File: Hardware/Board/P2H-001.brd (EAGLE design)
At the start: 47 x 72 mm, 14 parts, among them IC1 74LS07N, IC2 LTC485N

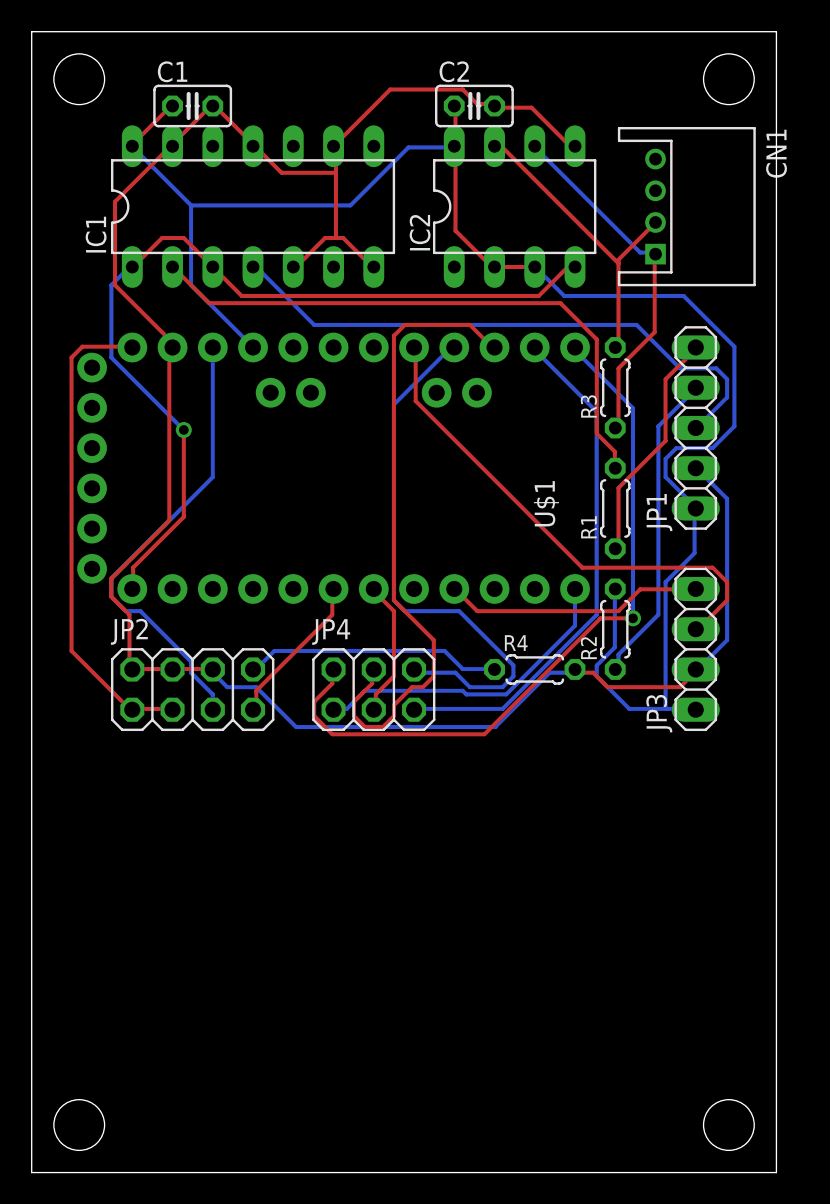
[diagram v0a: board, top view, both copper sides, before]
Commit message: New board design.
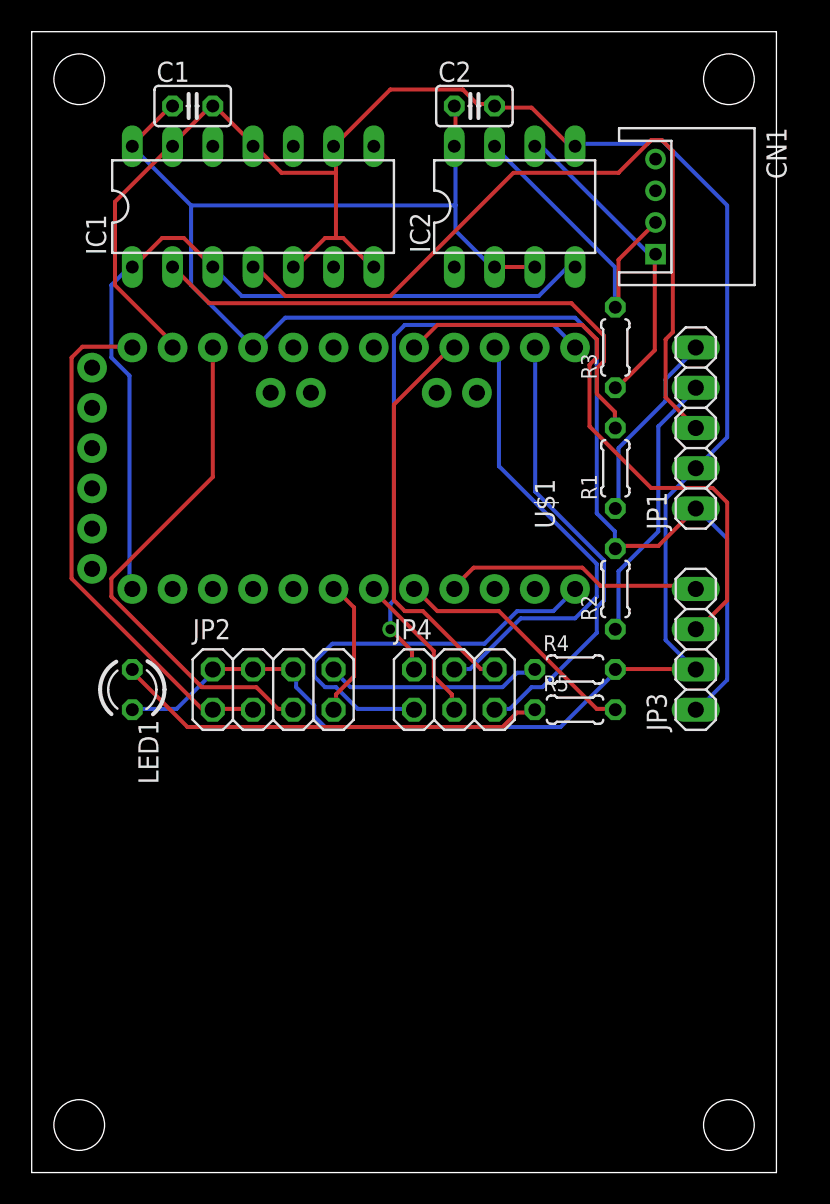
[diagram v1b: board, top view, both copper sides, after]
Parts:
- added LED1: (no value), led:LED3MM
- added R5: 330, resistor:0204/5
- moved JP4 5.08 mm to (26.7, 30.5)
- moved JP2 5.08 mm to (15.2, 30.5)
- moved R1 2.54 mm to (36.8, 44.5)
- moved R2 2.54 mm to (36.8, 36.8)
- moved R3 2.54 mm to (36.8, 52.1)
- moved R4 2.54 mm to (34.3, 31.8)
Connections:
- new net N$20: R5.2, U$1.8
- new net N$21: LED1.A, R5.1
- net GND: now also LED1.K
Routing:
- net N$21: track 0.00 -> 27.4 mm
- net N$20: track 0.00 -> 15.9 mm
- net N$4: track 36.8 -> 50.1 mm
- net N$13: track 45.7 -> 34.2 mm
- net N$15: track 40.2 -> 29.3 mm
- net N$17: track 34.7 -> 25.8 mm
- net GND: track 137.0 -> 144.2 mm
- net N$12: track 19.9 -> 26.5 mm
- net N$10: track 31.7 -> 37.8 mm
- net N$6: track 28.7 -> 32.8 mm
- net N$16: track 32.5 -> 28.5 mm
- net N$1: track 55.2 -> 52.5 mm, vias 1 -> 0
- net N$5: track 16.2 -> 13.6 mm
- net N$7: track 14.8 -> 12.3 mm
- net N$18: track 22.5 -> 20.0 mm
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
